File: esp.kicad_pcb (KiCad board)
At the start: 4 copper layers, 20 x 40.8 mm, 45 parts, among them J1 USB_C_Receptacle_USB2.0_14P, J2 Conn_01x04_Pin, SW1 RESET, SW2 BOOT, U1 ESP32-C3, U2 W25Q128JVP, U3 USBLC6-2P6, U4 MS5611-01BA, U5 SPX3819M5-L-3-3, U6 SHTC3, Y2 Crystal_GND24

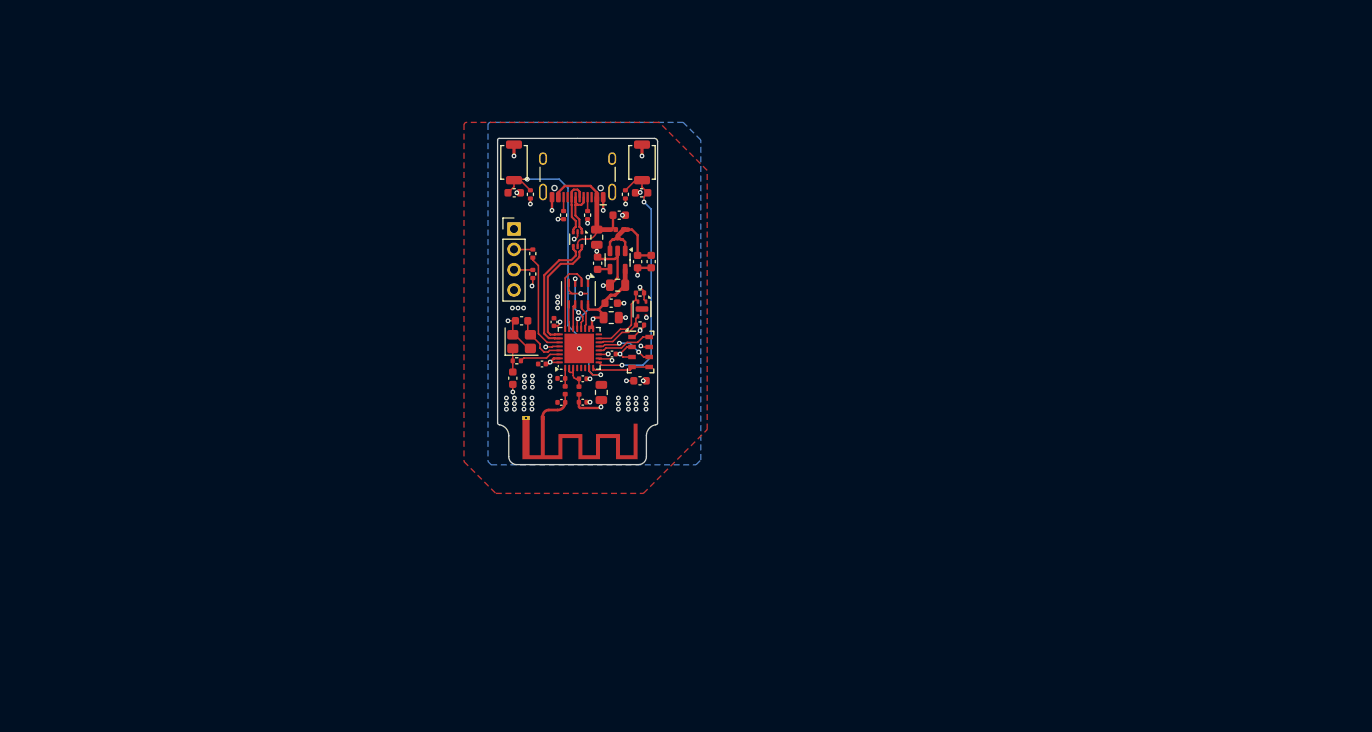
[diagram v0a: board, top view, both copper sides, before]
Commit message: pushing before redoing everything
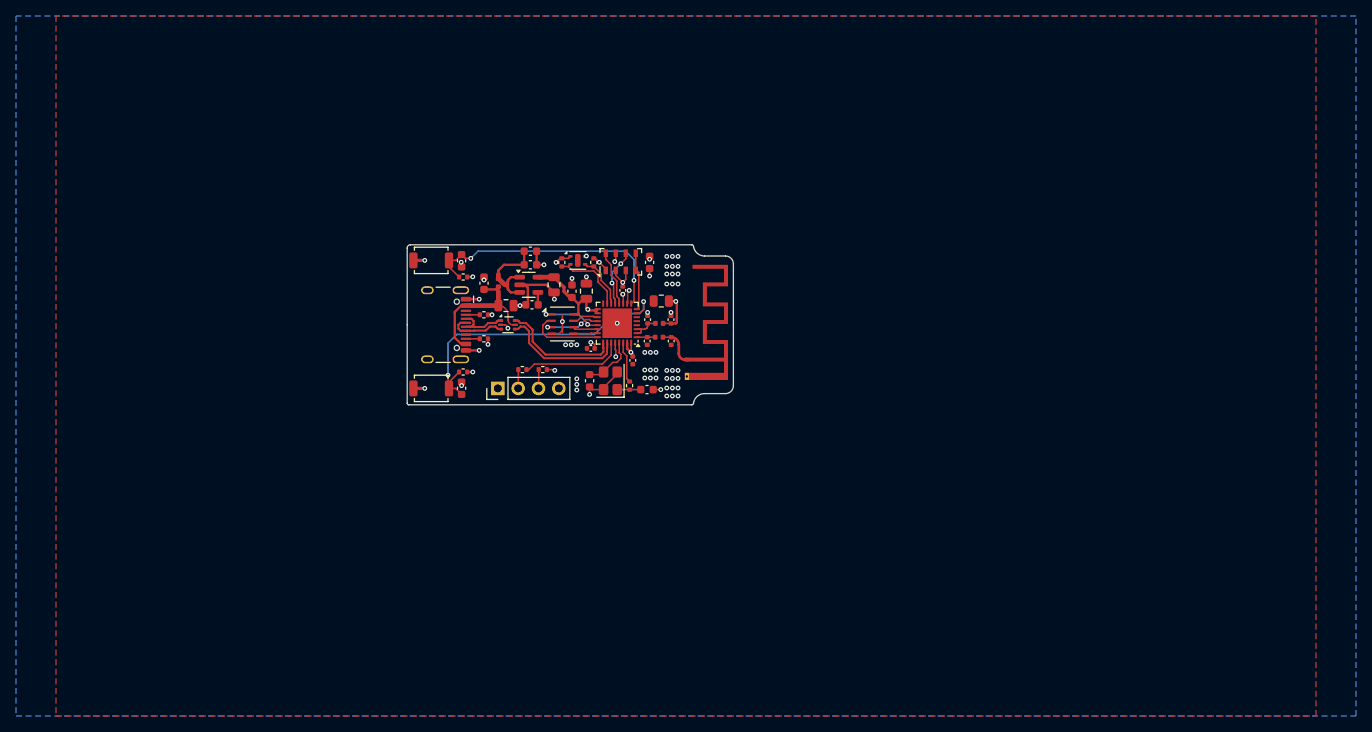
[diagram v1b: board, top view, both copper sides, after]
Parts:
- moved SW1 30.1 mm to (151.9, 69.0), turned to 0 degrees
- moved SW2 29.1 mm to (151.9, 53.0), turned to 0 degrees
- moved J1 26.5 mm to (152.5, 61.1), turned to -90 degrees
- moved C10 25.3 mm to (155.7, 69.0), turned to 90 degrees
- moved C18 24.1 mm to (155.7, 53.1), turned to -90 degrees
- moved R2 23.7 mm to (155.9, 67.0), turned to 180 degrees
- moved R7 22.8 mm to (155.9, 55.1), turned to 180 degrees
- moved J2 20.0 mm to (160.2, 69.0), turned to 90 degrees
- moved AE1 19.4 mm to (183.8, 65.5), turned to -90 degrees
- moved C13 18.9 mm to (158.5, 55.9), turned to 90 degrees
- moved R6 18.4 mm to (158.5, 62.9), turned to 0 degrees
- moved R5 18.0 mm to (158.5, 59.9), turned to 0 degrees
- moved C1 16.8 mm to (178.9, 69.2), turned to 0 degrees
- moved L2 16.5 mm to (160.3, 55.9), turned to 90 degrees
- moved C21 15.7 mm to (181.9, 63.1), turned to -90 degrees
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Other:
- board size 20 x 40.8 mm -> 40.8 x 20 mm
